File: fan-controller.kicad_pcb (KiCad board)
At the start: 2 copper layers, 34.5 x 20 mm, 25 parts, among them J1 PWR, J2 PTC, J3 FAN, J4 Conn_ARM_SWD_TagConnect_TC203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, Q1 AO3401A, Q2 MMBT5401, Q3 MMBT5551, Q4 MMBT5551, U1 L78L05, U2 PY32F002A

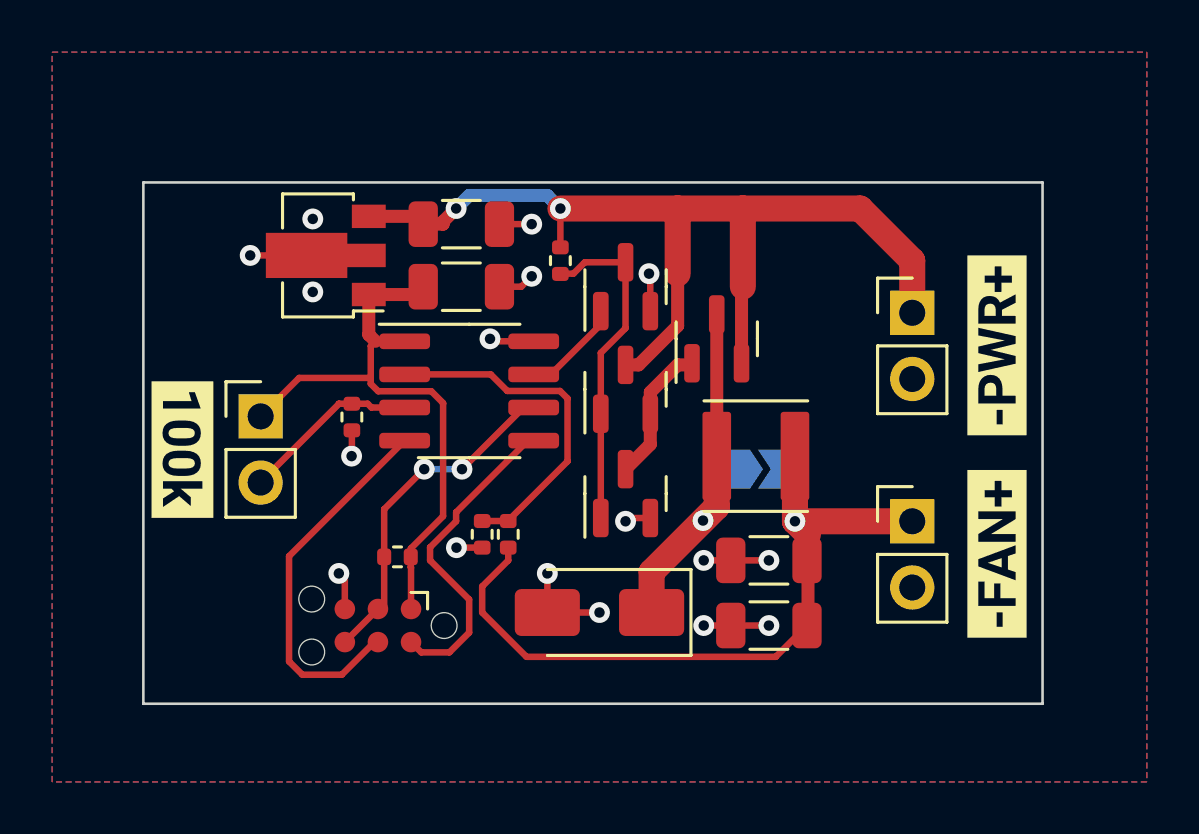
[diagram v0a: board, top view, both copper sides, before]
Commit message: Simplify circuit
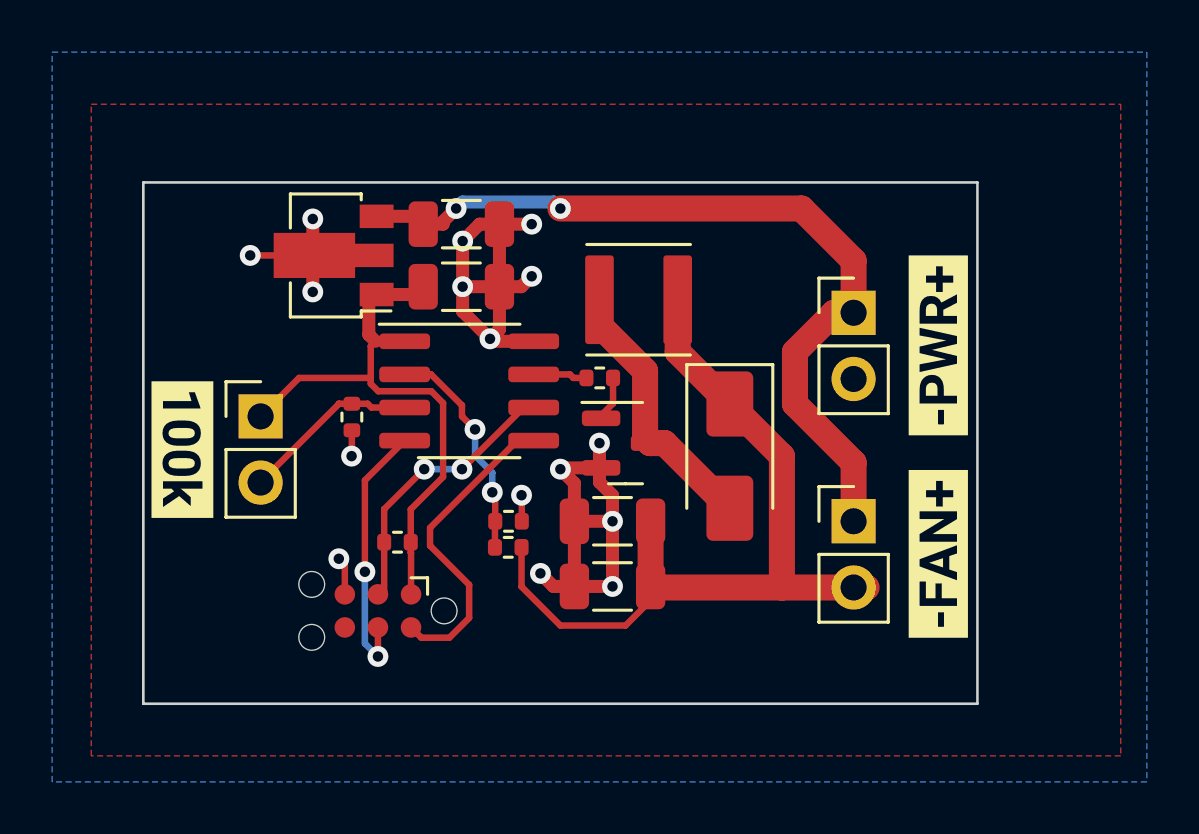
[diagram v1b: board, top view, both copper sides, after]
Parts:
- removed JP1: PWM_MODE, Jumper:SolderJumper-2_P1.3mm_Open_TrianglePad1.0x1.5mm
- removed Q1: AO3401A, Package_TO_SOT_SMD:SOT-23
- removed Q2: MMBT5401, Package_TO_SOT_SMD:SOT-23
- removed Q3, Q4: MMBT5551, Package_TO_SOT_SMD:SOT-23
- removed R7: 22k, Resistor_SMD:R_0402_1005Metric
- added Q5: AO3400A, Package_TO_SOT_SMD:SOT-23, F.Cu at (117.0, 62.0)
- added R5: 100, Resistor_SMD:R_0402_1005Metric, F.Cu at (116.0, 59.5)
- R2: value 22k -> 100k
- R3: value 100k -> 22k
- moved D1 7.81 mm to (121.0, 62.5), turned to -90 degrees
- moved L1 7.50 mm to (117.5, 56.5)
- moved C3 6.18 mm to (116.5, 67.5)
- moved C4 6.18 mm to (116.5, 65.0)
- moved J1 2.25 mm to (125.8, 57.0)
- moved J3 2.25 mm to (125.8, 65.0)
- moved kibuzzard-1 2.25 mm to (129.0, 58.2)
- moved kibuzzard-3 2.25 mm to (129.0, 66.2)
- moved R2 1.12 mm to (112.5, 66.0), turned to 180 degrees
- moved J4 0.56 mm to (107.5, 68.4)
- moved R4 0.56 mm to (108.2, 65.8)
- moved R3 0.50 mm to (112.5, 65.0), turned to 180 degrees
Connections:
- C3 pad 1: /FAN_OUT -> /FAN_OUT-
- C4 pad 1: /FAN_OUT -> /FAN_OUT-
- D1 pad 1: Net-(D1-K) -> /FAN_OUT-
- D1 pad 2: GND -> Net-(D1-A)
- J3 pad 1: /FAN_OUT -> VPP
- J3 pad 2: GND -> /FAN_OUT-
- J4 pad 6: /~{RST} -> unconnected-(J4-SWO-Pad6)
- L1 pad 1: Net-(D1-K) -> Net-(D1-A)
- L1 pad 2: /FAN_OUT -> /FAN_OUT-
- R2 pad 1: /FAN_SENSE -> /FAN_OUT-
- R2 pad 2: GND -> Net-(U2-PA4/PA10)
- R3 pad 1: /FAN_OUT -> GND
- R3 pad 2: /FAN_SENSE -> Net-(U2-PA4/PA10)
- U2 pad 2: /FAN_SENSE -> Net-(U2-PA4/PA10)
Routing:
- net /FAN_OUT-: track 0.00 -> 30.4 mm
- net /FAN_OUT: track 29.6 -> 0.00 mm, vias 1 -> 0
- net GND: track 23.2 -> 47.5 mm, vias 17 -> 16
- net Net-(D1-K): track 15.0 -> 0.00 mm, vias 1 -> 0
- net /FAN_SENSE: track 13.3 -> 0.00 mm
- net Net-(Q2-B): track 12.9 -> 0.00 mm
- net Net-(D1-A): track 0.00 -> 9.39 mm
- net Net-(U2-PA4/PA10): track 0.00 -> 8.65 mm, vias 0 -> 2
- net VPP: track 38.6 -> 31.7 mm
- net Net-(Q1-G): track 5.33 -> 0.00 mm
- net /SWCLK: track 14.5 -> 10.2 mm, vias 0 -> 2
- net /~{RST}: track 12.5 -> 10.1 mm
- net Net-(Q5-G): track 0.00 -> 1.72 mm
- net /SWDIO: track 12.2 -> 11.4 mm
- net +5V: track 23.1 -> 22.6 mm
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- added copper zone on F.Cu, net (none)
- removed copper zone on F.Cu, net GND
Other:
- board size 34.5 x 20 mm -> 32 x 20 mm
- board text added: "flaviutamas.com/p/fan-temp 5-24V Fan Temp Controller Ifan≤300mA"
- board text removed: "flaviutamas.com/p/dc-fan-temp 5-24V Fan Temp Controller Ifan≤250mA"
